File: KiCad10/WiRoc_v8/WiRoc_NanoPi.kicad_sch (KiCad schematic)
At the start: 49 parts, among them J10 Conn_01x09_Socket, J12 TC2050, J2 Conn_01x04, J5 Conn_01x04_Socket, J6 HAT_Conn_DBG, J8 Conn_01x06, SW1 SW_SPST, U1 SY6280, U10 SY7069ADC, U2 OLED, U3 AXP209, U5 SY6280, U6 BatteryPadM, U7 BatteryPadP

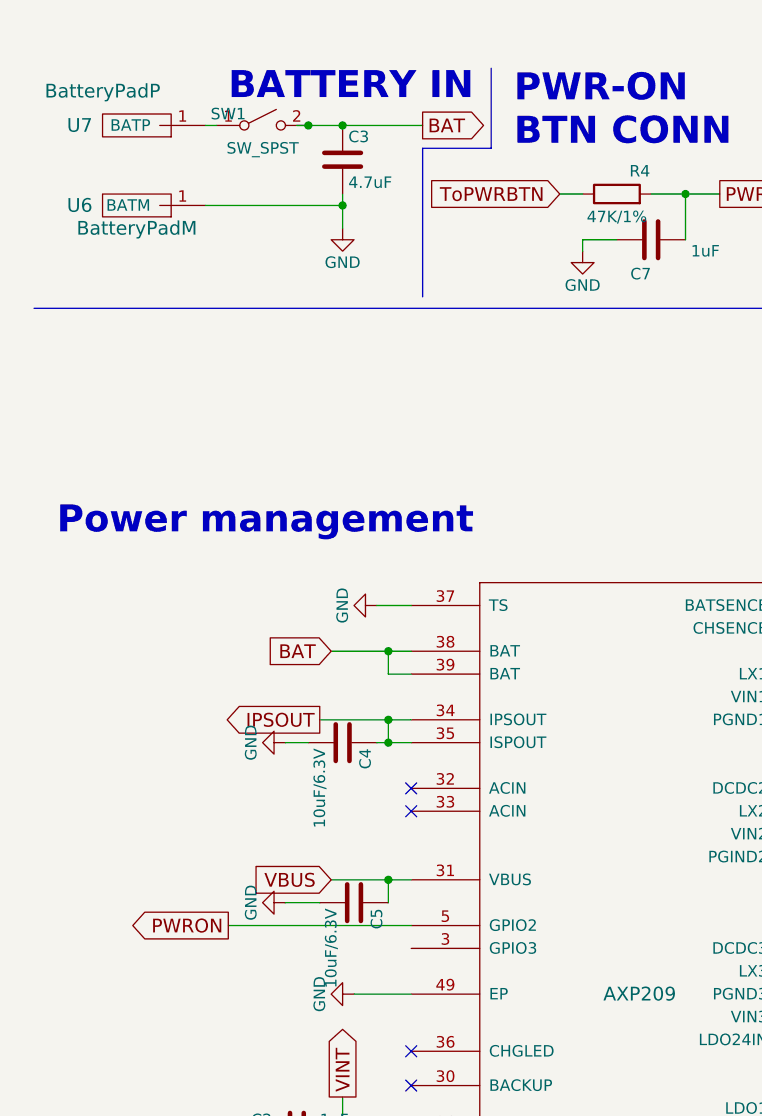
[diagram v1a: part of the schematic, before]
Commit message: etc
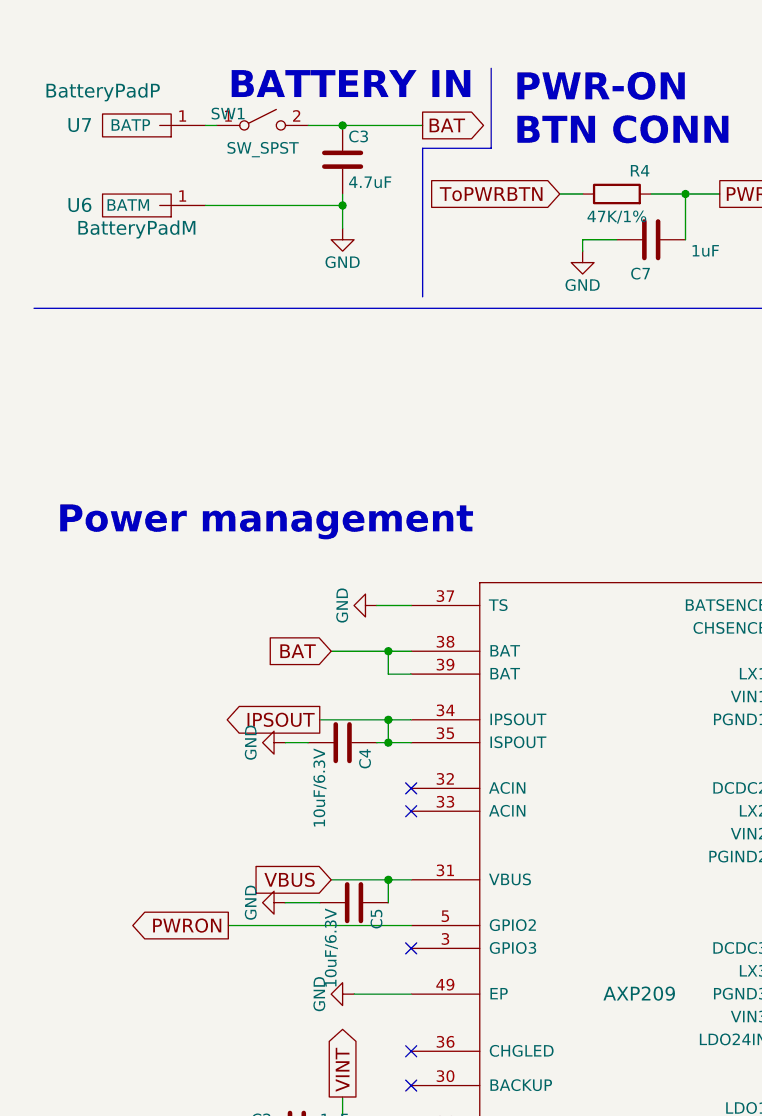
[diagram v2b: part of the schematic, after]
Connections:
- no-connect marks 26 -> 27
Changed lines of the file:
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@@
-	)
-	(junction
-		(at 43.18 20.32)
-		(diameter 0)
-		(color 0 0 0 0)
 	)
 	(junction
@@
 		(at 137.16 38.1)
 	)
+	(no_connect
+		(at 54.61 111.76)
+	)
 	(polyline
 		(pts
@@
 		)
 		(stroke
-			(width 0)
-			(type default)
-		)
-	)
-	(wire
-		(pts
-			(xy 41.91 20.32) (xy 43.18 20.32)
-		)
-		(stroke
